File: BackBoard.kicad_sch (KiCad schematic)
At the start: 81 parts, among them J14 Power to TopBoard, J15 Comm to TopBoard, J16 Conn_01x08_Socket, J17 ST-Link, J18 ST-Link, M1 STS3032, M2 STS3032, M3 STS3032, M4 STS3032, Q3 TJ15S06M3L, Q4 BSS138, Q5 BSS138, SW3 B-12CCP, SW4 RESET_SWITCH, SW5 MODE_SWITCH, SW6 B-12CCP, SW7 RESET_SWITCH, SW8 MODE_SWITCH, U10 AZ1117CH-3.3TRG1, U12 AE-BNO055-BO, U14 STM32F446RET6, U15 Sit2001B, U16 STM32F446RET6, U17 Sit2001B, U18 MAX3485, U9 MIC5219-5.0YM5-TR

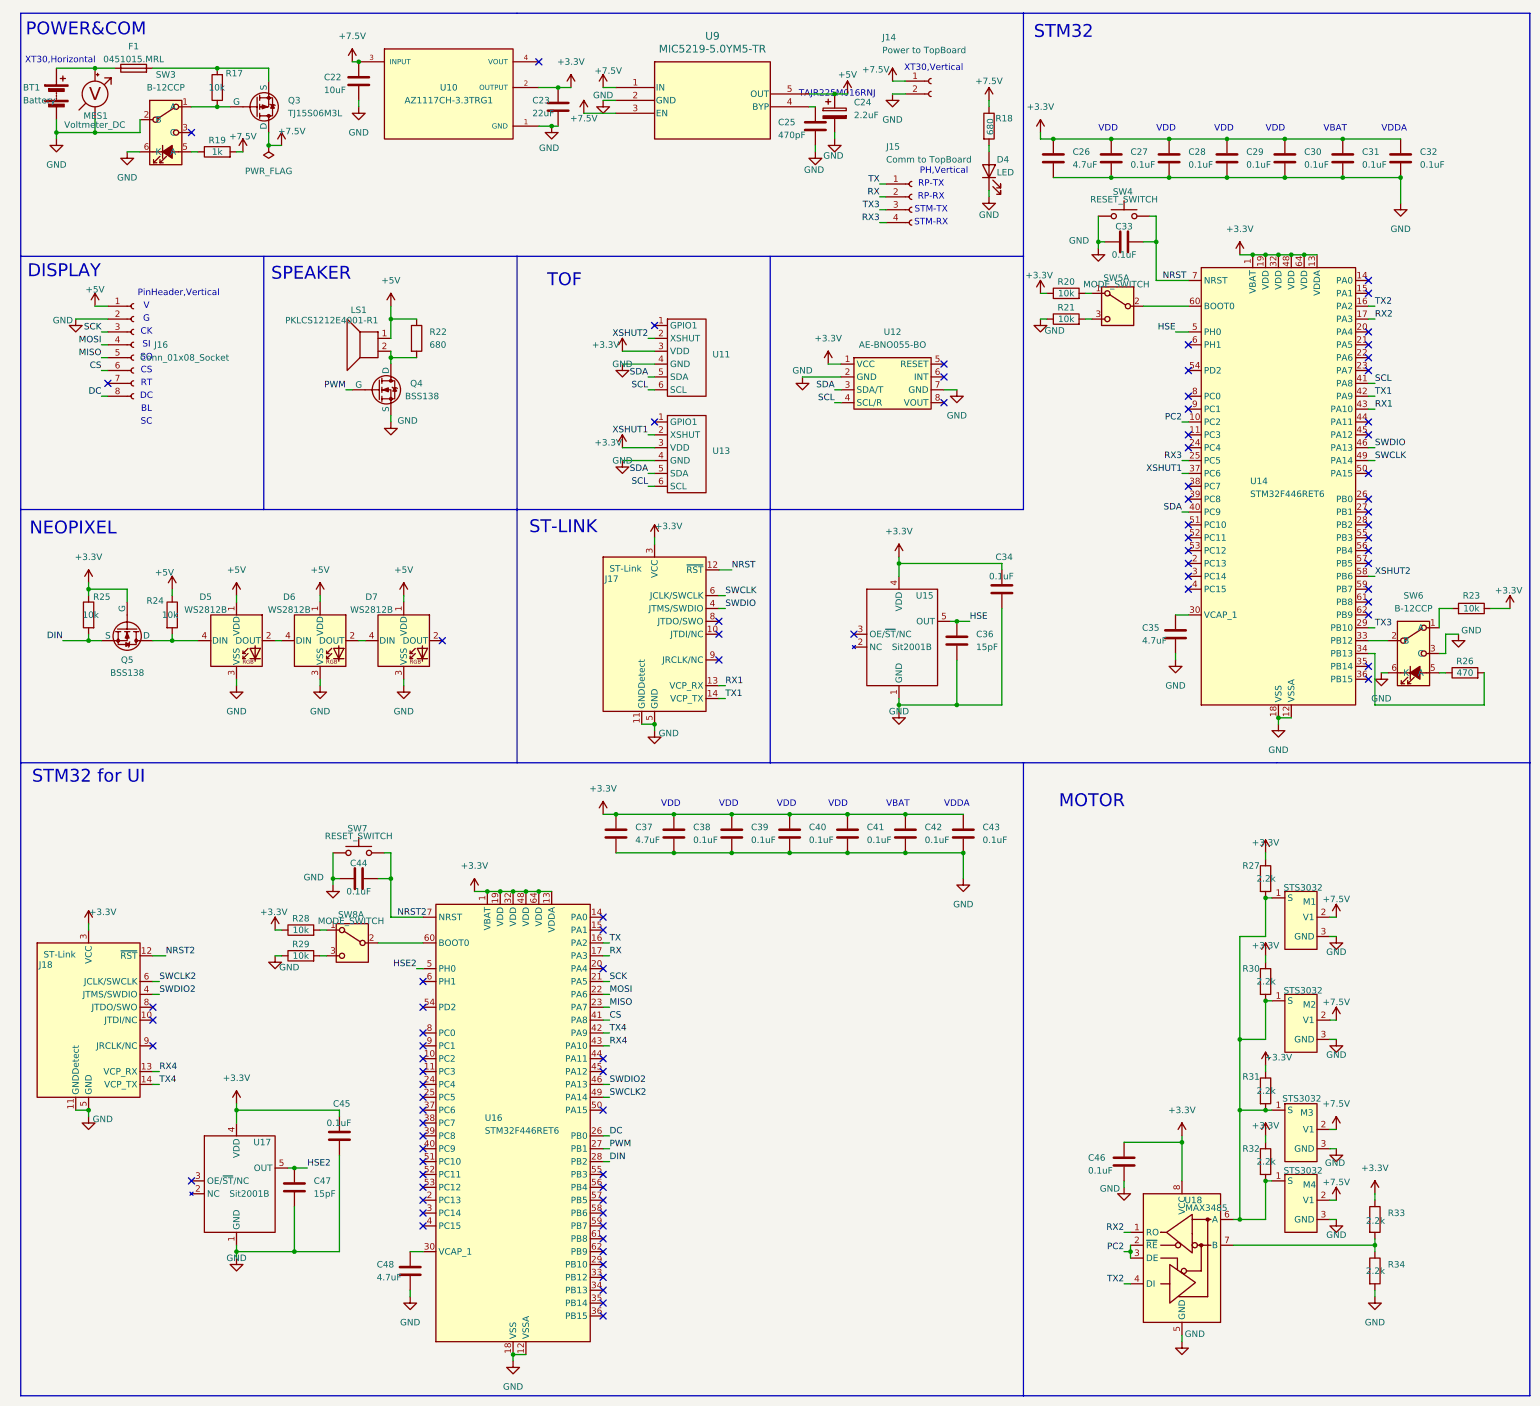
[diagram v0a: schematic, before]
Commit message: メイン基板Rev.3
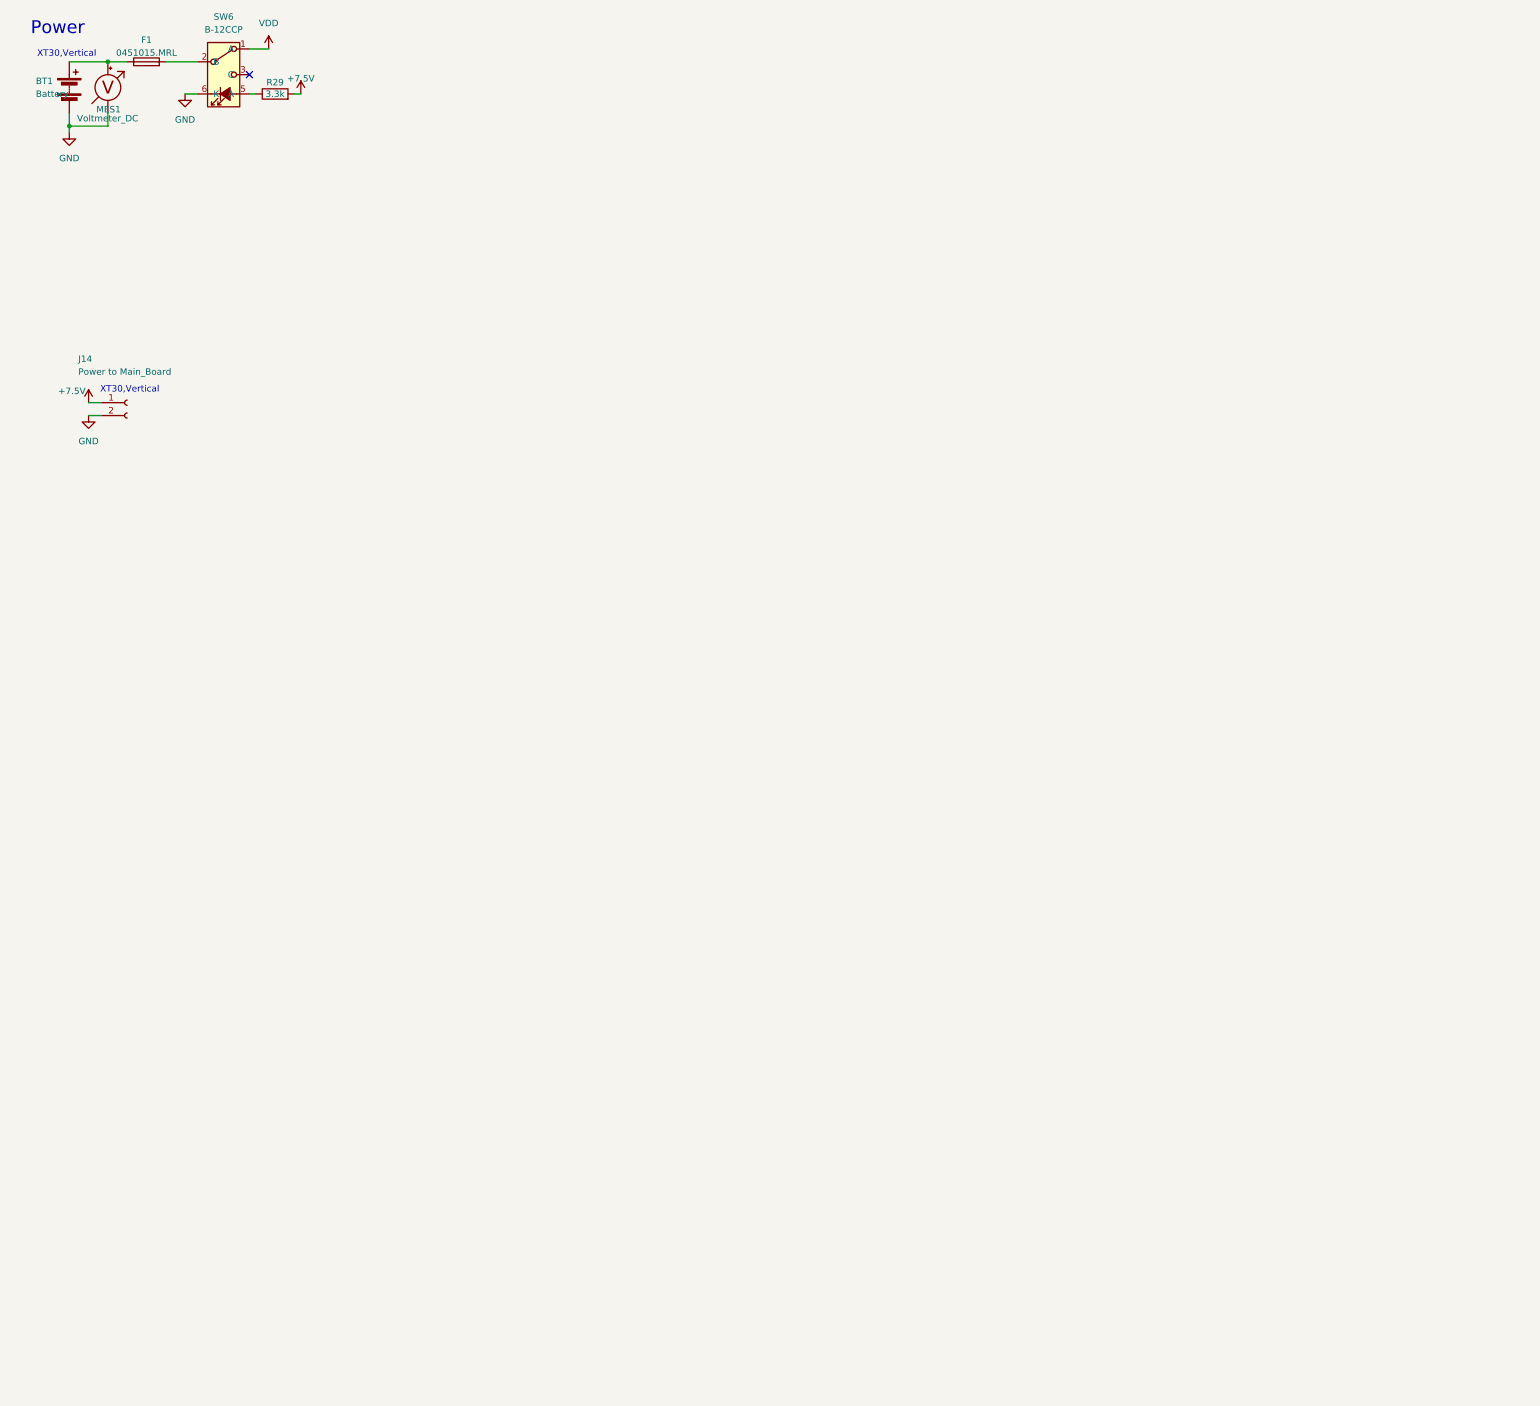
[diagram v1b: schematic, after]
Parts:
- removed C22: 10uF, Capacitor_SMD:C_0603_1608Metric_Pad1.08x0.95mm_HandSolder, symbol Device:C
- removed C23: 22uF, Capacitor_SMD:C_0603_1608Metric_Pad1.08x0.95mm_HandSolder, symbol Device:C
- removed C24: 2.2uF, Capacitor_SMD:C_0805_2012Metric, symbol Device:C_Polarized
- removed C25: 470pF, Capacitor_SMD:C_0603_1608Metric_Pad1.08x0.95mm_HandSolder, symbol Device:C
- removed C26, C35, C37, C48: 4.7uF, Capacitor_SMD:C_0603_1608Metric_Pad1.08x0.95mm_HandSolder, symbol Device:C
- removed C27, C28, C29, C30, C31, C32, C33, C34, C38, C39, C40, C41, C42, C43, C44, C45, C46: 0.1uF, Capacitor_SMD:C_0603_1608Metric_Pad1.08x0.95mm_HandSolder, symbol Device:C
- removed C36, C47: 15pF, Capacitor_SMD:C_0603_1608Metric_Pad1.08x0.95mm_HandSolder, symbol Device:C
- removed D4: LED, LED_SMD:LED_0603_1608Metric, symbol Device:LED
- removed D5, D6, D7: WS2812B, LED_SMD:LED_WS2812B_PLCC4_5.0x5.0mm_P3.2mm, symbol LED:WS2812B
- removed J15: Comm to TopBoard, Connector_JST:JST_PH_B4B-PH-K_1x04_P2.00mm_Vertical, symbol Connector:Conn_01x04_Socket
- removed J16: Conn_01x08_Socket, Connector_PinSocket_2.54mm:PinSocket_1x08_P2.54mm_Vertical, symbol Connector:Conn_01x08_Socket
- removed J17, J18: ST-Link, STDC14:CONN14_3220-14_CNC, symbol Connector:Conn_ST_STDC14
- removed LS1: PKLCS1212E4001-R1, PKLCS1212E4001-R1:PKLCS1212E4001R1, symbol Device:Speaker
- removed M1, M2, M3, M4: STS3032, Connector_JST:JST_XH_B3B-XH-A_1x03_P2.50mm_Vertical, symbol STS3032:STS3032
- removed Q3: TJ15S06M3L, Package_TO_SOT_SMD:TO-252-2, symbol Simulation_SPICE:PMOS
- removed Q4, Q5: BSS138, Package_TO_SOT_SMD:SOT-23, symbol Simulation_SPICE:NMOS
- removed R17: 10k, Resistor_SMD:R_0603_1608Metric, symbol Device:R
- removed R18, R22: 680, Resistor_SMD:R_0603_1608Metric, symbol Device:R
- removed R19: 1k, Resistor_SMD:R_0603_1608Metric, symbol Device:R
- removed R20, R21, R23, R24, R25, R28: 10k, Capacitor_SMD:C_0603_1608Metric_Pad1.08x0.95mm_HandSolder, symbol Device:R
- removed R26: 470, Resistor_SMD:R_0603_1608Metric, symbol Device:R
- removed R27, R30, R31, R32, R33, R34: 2.2k, Capacitor_SMD:C_0603_1608Metric_Pad1.08x0.95mm_HandSolder, symbol Device:R
- removed SW3: B-12CCP, B-12CCP:B-12CCP, symbol B-12CCP:B-12CCP
- removed SW4, SW7: RESET_SWITCH, SKRPACE010:SW_SKRPACE010, symbol Switch:SW_Push
- removed SW5, SW8: MODE_SWITCH, SSSS213202:SSSS213202, symbol Switch:SW_DPDT_x2
- removed U10: AZ1117CH-3.3TRG1, AZ1117CH-3.3TRG1:DIODES_AZ1117CH-3.3TRG1_0, symbol AZ1117CH:AZ1117CH-3.3TRG1
- removed U11, U13: ~, Connector_PinSocket_2.54mm:PinSocket_1x06_P2.54mm_Vertical, symbol VL53l0X:VL53L0X_SwScience_6pin
- removed U12: AE-BNO055-BO, AE-BNO055-BO:AE-BNO055-BO, symbol AE-BNO055-BO:AE-BNO055-BO
- removed U14, U16: STM32F446RET6, Package_QFP:LQFP-64_10x10mm_P0.5mm, symbol MCU_ST_STM32F4:STM32F446RETx
- removed U15, U17: Sit2001B, Package_TO_SOT_SMD:SOT-23-5, symbol SiT2001B:Sit2001B
- removed U18: MAX3485, Package_SO:SOIC-8_3.9x4.9mm_P1.27mm, symbol Interface_UART:MAX3485
- removed U9: MIC5219-5.0YM5-TR, Package_TO_SOT_SMD:SOT-23-5, symbol MIC5219-5.0YM5-TR:MIC5219-5.0YM5-TR
- BT1: footprint Connector_AMASS:AMASS_XT30PW-F_1x02_P2.50mm_Horizontal -> Connector_AMASS:AMASS_XT30U-M_1x02_P5.0mm_Vertical
- J14: value Power to TopBoard -> Power to Main_Board; footprint Connector_AMASS:AMASS_XT30U-F_1x02_P5.0mm_Vertical -> Connector_AMASS:AMASS_XT30U-M_1x02_P5.0mm_Vertical
- R29: value 10k -> 3.3k; footprint Capacitor_SMD:C_0603_1608Metric_Pad1.08x0.95mm_HandSolder -> Resistor_SMD:R_0603_1608Metric
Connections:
- net +7.5V: now also R29.2
- net GND: no longer R29.1, SW6.3 (C)
- net at F1.2: now also SW6.2 (B)
- net VDD: now reaches SW6.1 (A)
- net at SW6.5 (A): now also R29.1
- no-connect marks 87 -> 1
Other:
- note added: "Power"
- note removed: "BL"
- note removed: "CK"
- note removed: "CS"
- note removed: "DC"
- note removed: "DISPLAY"
- note removed: "G"
- note removed: "MOTOR"
- note removed: "NEOPIXEL"
- note removed: "PH,Vertical"
- note removed: "POWER&COM"
- note removed: "PinHeader,Vertical"
- note removed: "RP-RX"
- note removed: "RP-TX"
- note removed: "RT"
- note removed: "SC"
- note removed: "SI"
- note removed: "SO"
- note removed: "SPEAKER"
- note removed: "ST-LINK"
- note removed: "STM-RX"
- note removed: "STM-TX"
- note removed: "STM32"
- note removed: "STM32 for UI"
- note removed: "TAJR225M016RNJ"
- note removed: "TOF"
- note removed: "V"
- note removed: "VBAT"
- note removed: "VDD"
- note removed: "VDDA"
- note removed: "XT30,Horizontal"
- company: Fornax -> (none)
- title: BackBoard Rev.2 -> (none)
